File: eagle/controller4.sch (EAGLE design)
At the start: 23 parts, among them K1 SRD-05VDC-SL-C, K2 SRD-05VDC-SL-C, K3 SRD-05VDC-SL-C, K4 SRD-05VDC-SL-C, T1 BC547, T2 BC547, T3 BC547, T4 BC547, X1 VCC, X2 IN1, X3 IN2, X4 IN3, X5 IN4

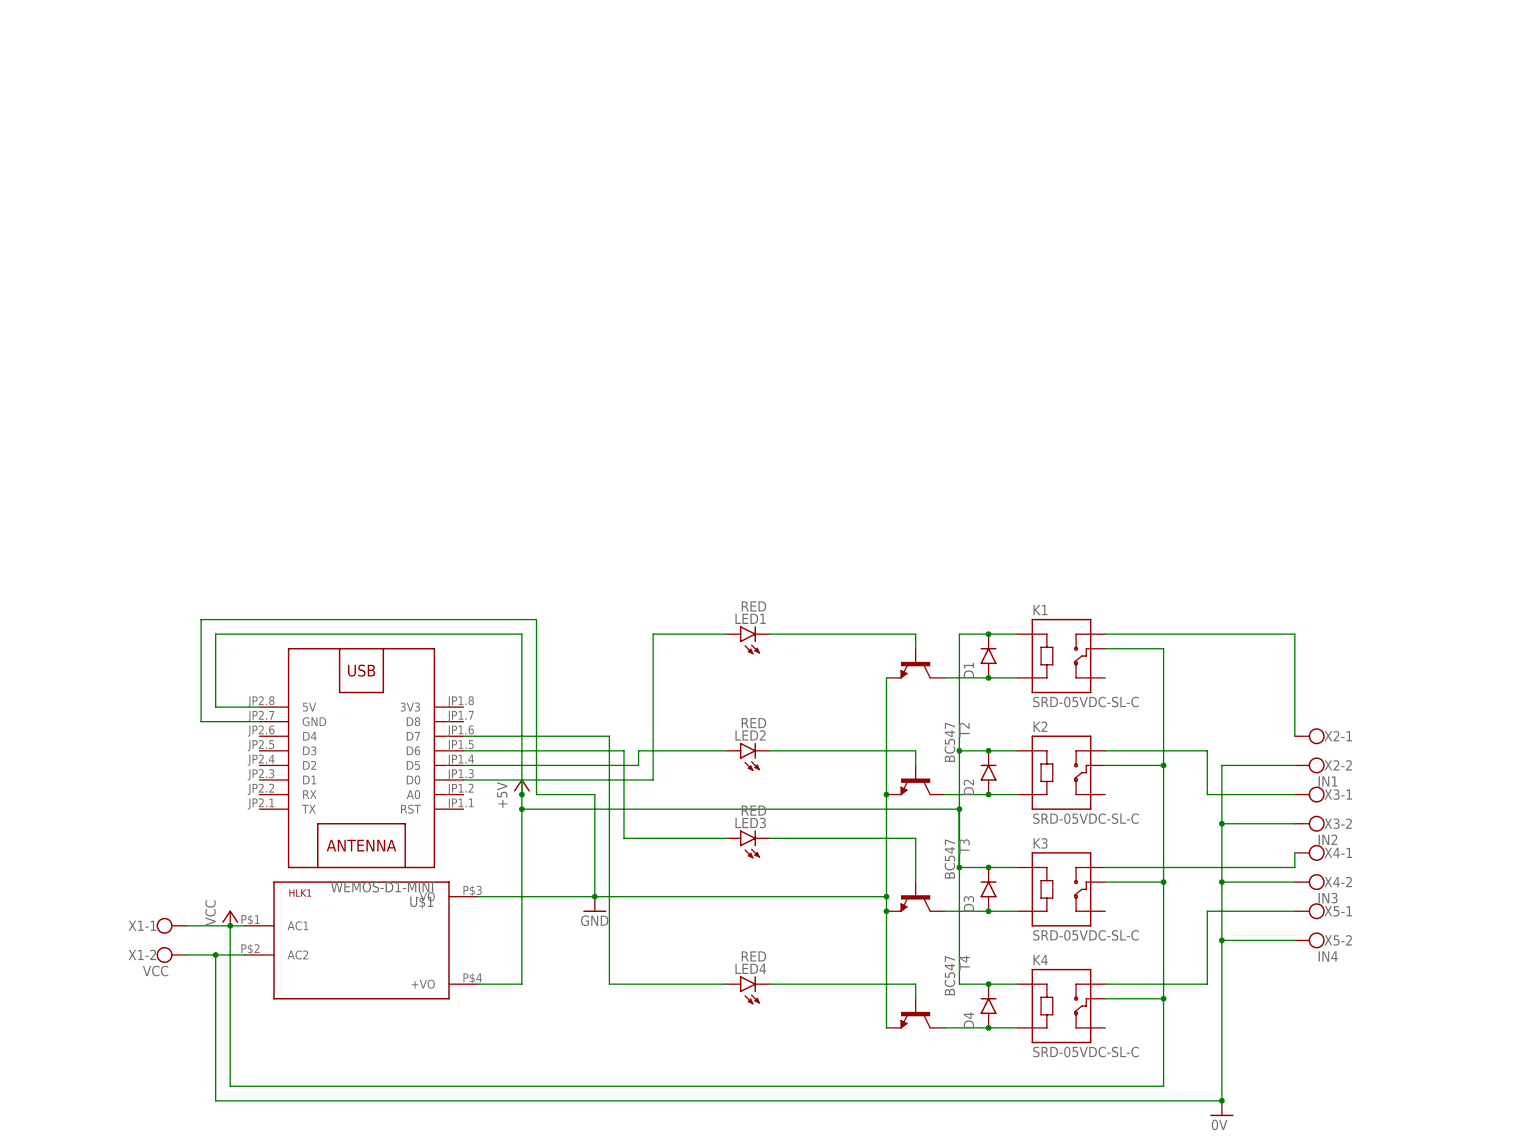
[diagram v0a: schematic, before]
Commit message: refactoring
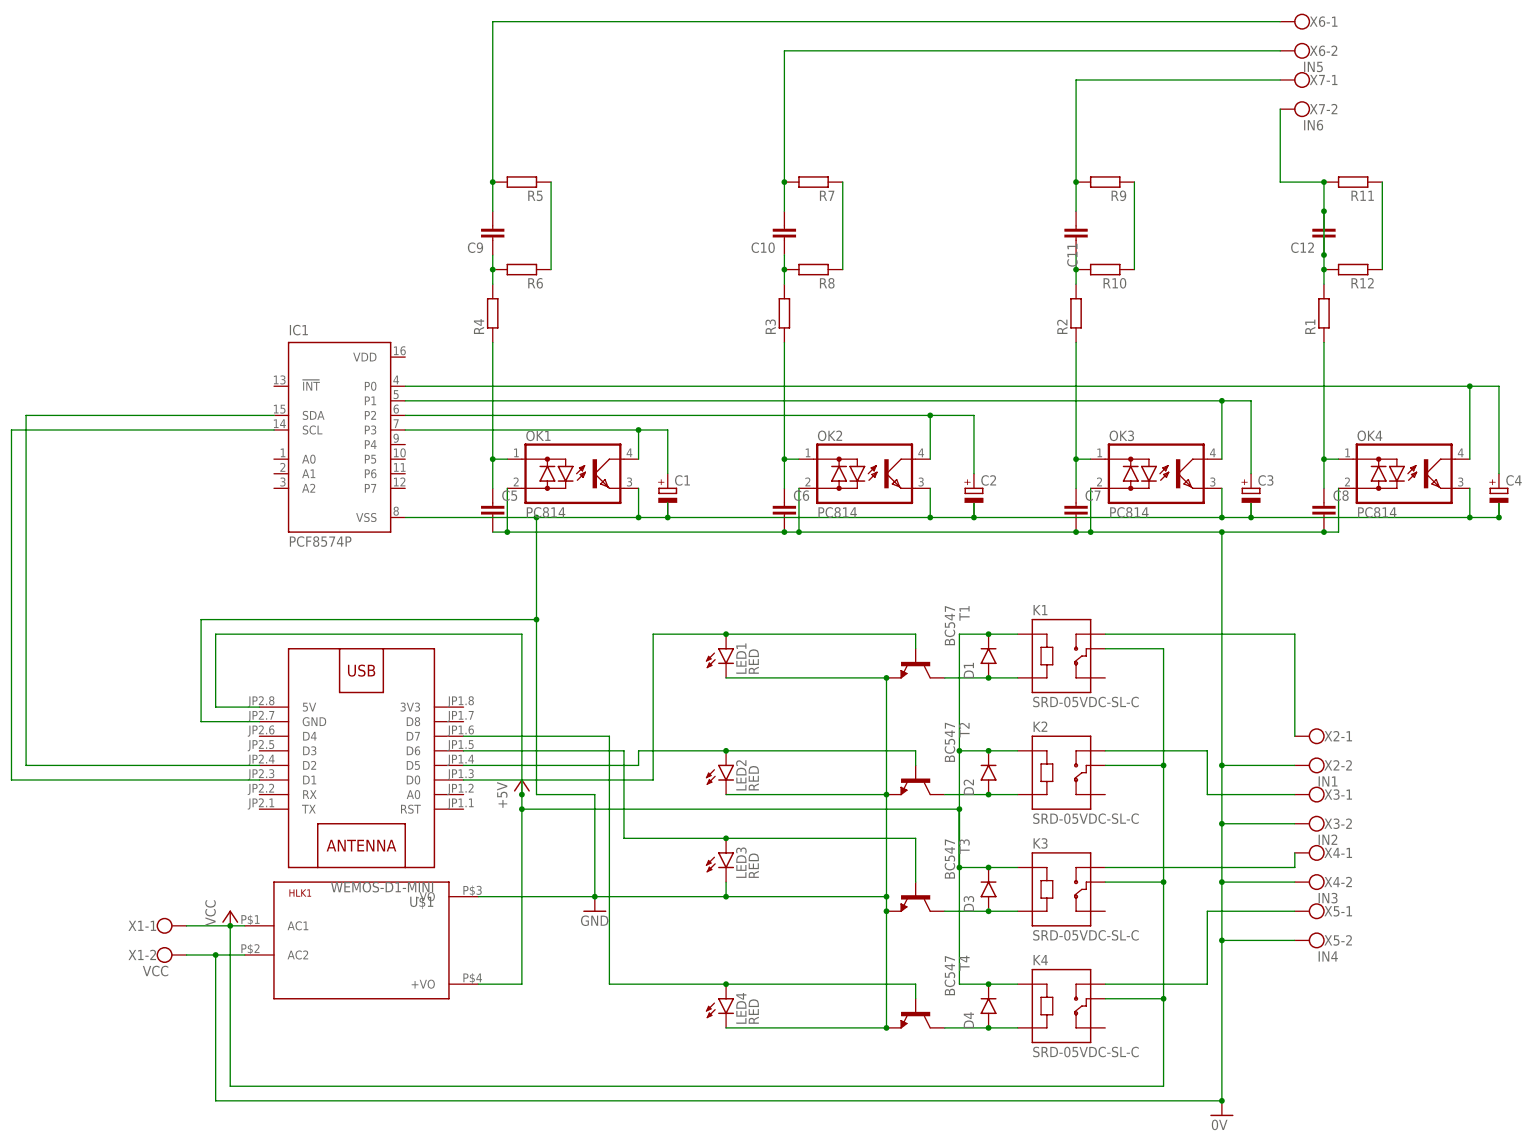
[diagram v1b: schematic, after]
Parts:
- added C1, C2, C3, C4: (no value), rcl:CPOL-EUE5-5
- added C10, C11, C12, C5, C6, C7, C8, C9: (no value), rcl:C-EU025-024X044
- added IC1: PCF8574P, micro-philips:PCF8574P
- added OK1, OK2, OK3, OK4: PC814, optocoupler:PC814
- added R1, R10, R11, R12, R2, R3, R4, R5, R6, R7, R8, R9: (no value), rcl:R-EU_0204/5
- added X6: IN5, con-wago-500:W237-102
- added X7: IN6, con-wago-500:W237-102
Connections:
- new net N$10: C9.1, R4.2, R6.2
- new net N$17: IC1.SCL, U$1.D1
- new net N$18: IC1.SDA, U$1.D2
- new net N$20: C10.1, R3.2, R8.2
- new net N$21: C11.1, R10.2, R2.2
- new net N$22: C8.1, OK4.AC1, R1.1
- new net N$23: C11.2, R9.2, X7-1.KL
- new net N$24: C10.2, R7.2, X6-2.KL
- new net N$25: C9.2, R5.2, X6-1.KL
- new net N$26: R5.1, R6.1
- new net N$27: C12.1, C12.2, R1.2, R11.2, R12.2, X7-2.KL
- new net N$28: C7.1, OK3.AC1, R2.1
- new net N$29: C6.1, OK2.AC1, R3.1
- new net N$30: C5.1, OK1.AC1, R4.1
- new net N$31: R7.1, R8.1
- new net N$32: R10.1, R9.1
- new net N$33: R11.1, R12.1
- net 0V: now also C5.2, C6.2, C7.2, C8.2, OK1.AC2, OK2.AC2, OK3.AC2, OK4.AC2
- net GND: now also C1.-, C2.-, C3.-, C4.-, IC1.VSS, LED1.C, LED2.C, LED3.C, LED4.C, OK1.E, OK2.E, OK3.E, OK4.E
- net N$14: now also T2.B
- net N$15: now also T1.B
- net N$16: now also T4.B
- net N$19: now also T3.B
- net N$6: now also C1.+, IC1.P3, OK1.C; no longer LED4.C, T4.B
- net N$7: now also C2.+, IC1.P2, OK2.C; no longer LED3.C, T3.B
- net N$8: now also C3.+, IC1.P1, OK3.C; no longer LED2.C, T2.B
- net N$9: now also C4.+, IC1.P0, OK4.C; no longer LED1.C, T1.B
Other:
- moved on the sheet: LED1, LED2, LED3, LED4
